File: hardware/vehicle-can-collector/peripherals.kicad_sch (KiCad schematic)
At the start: 16 parts, among them J301 Micro_SD_Card_Det, J302 USB_B_Micro, J303 I2C_STANDARD, U301 FT2232HL, U302 93C56B

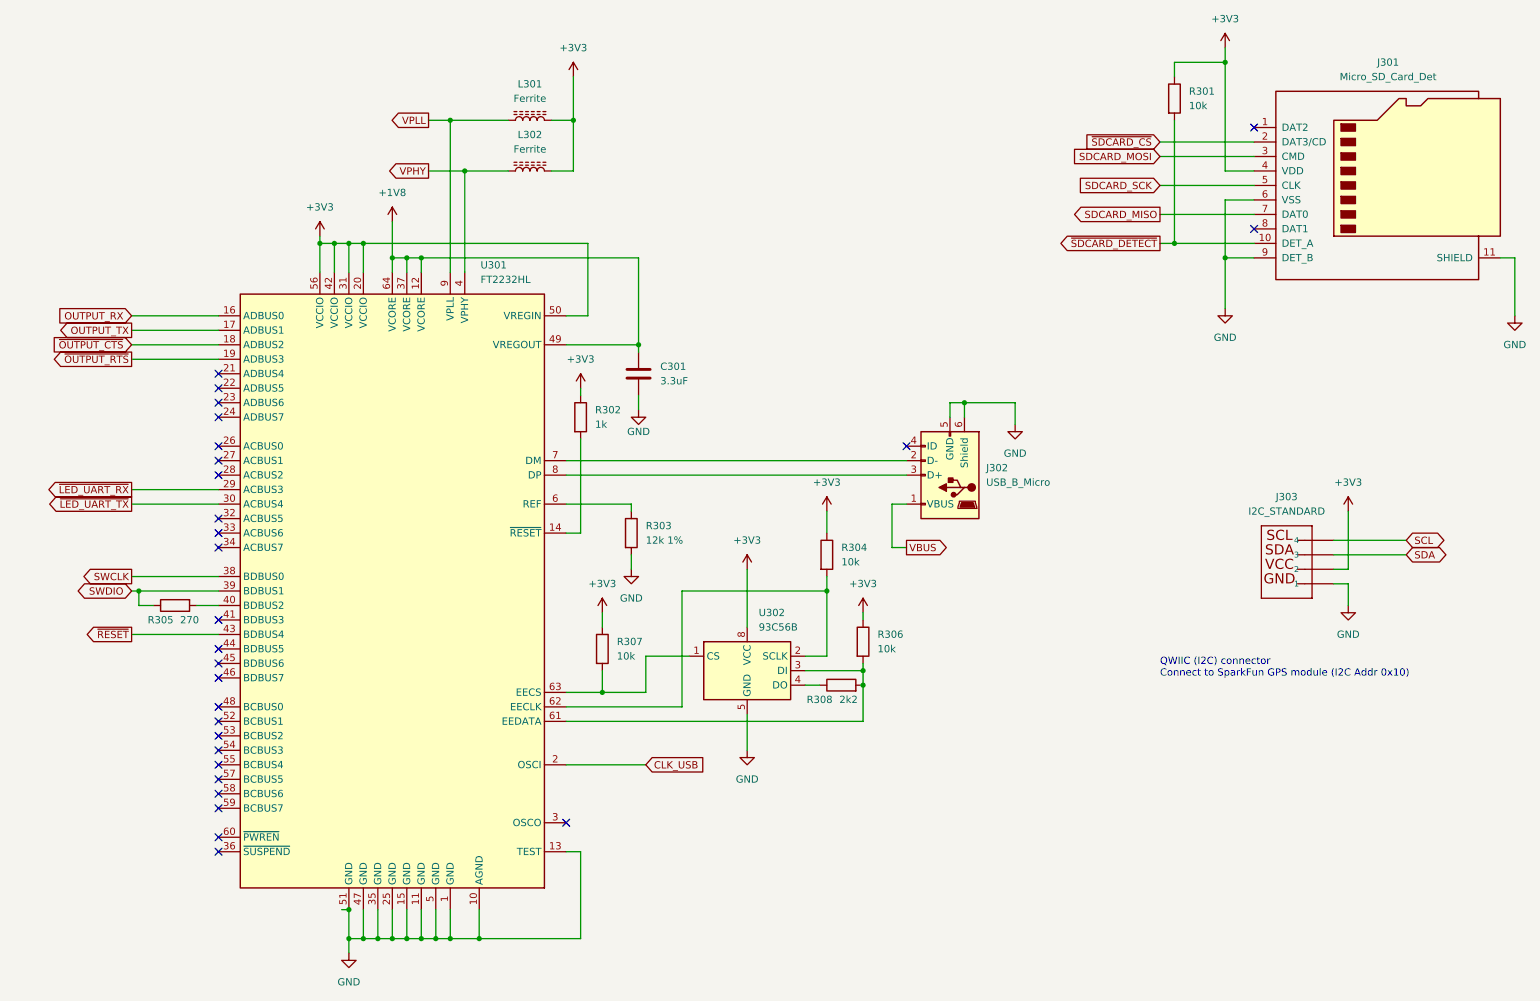
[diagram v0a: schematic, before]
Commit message: Finished first round of layout.
- dang this has a lot of parts!
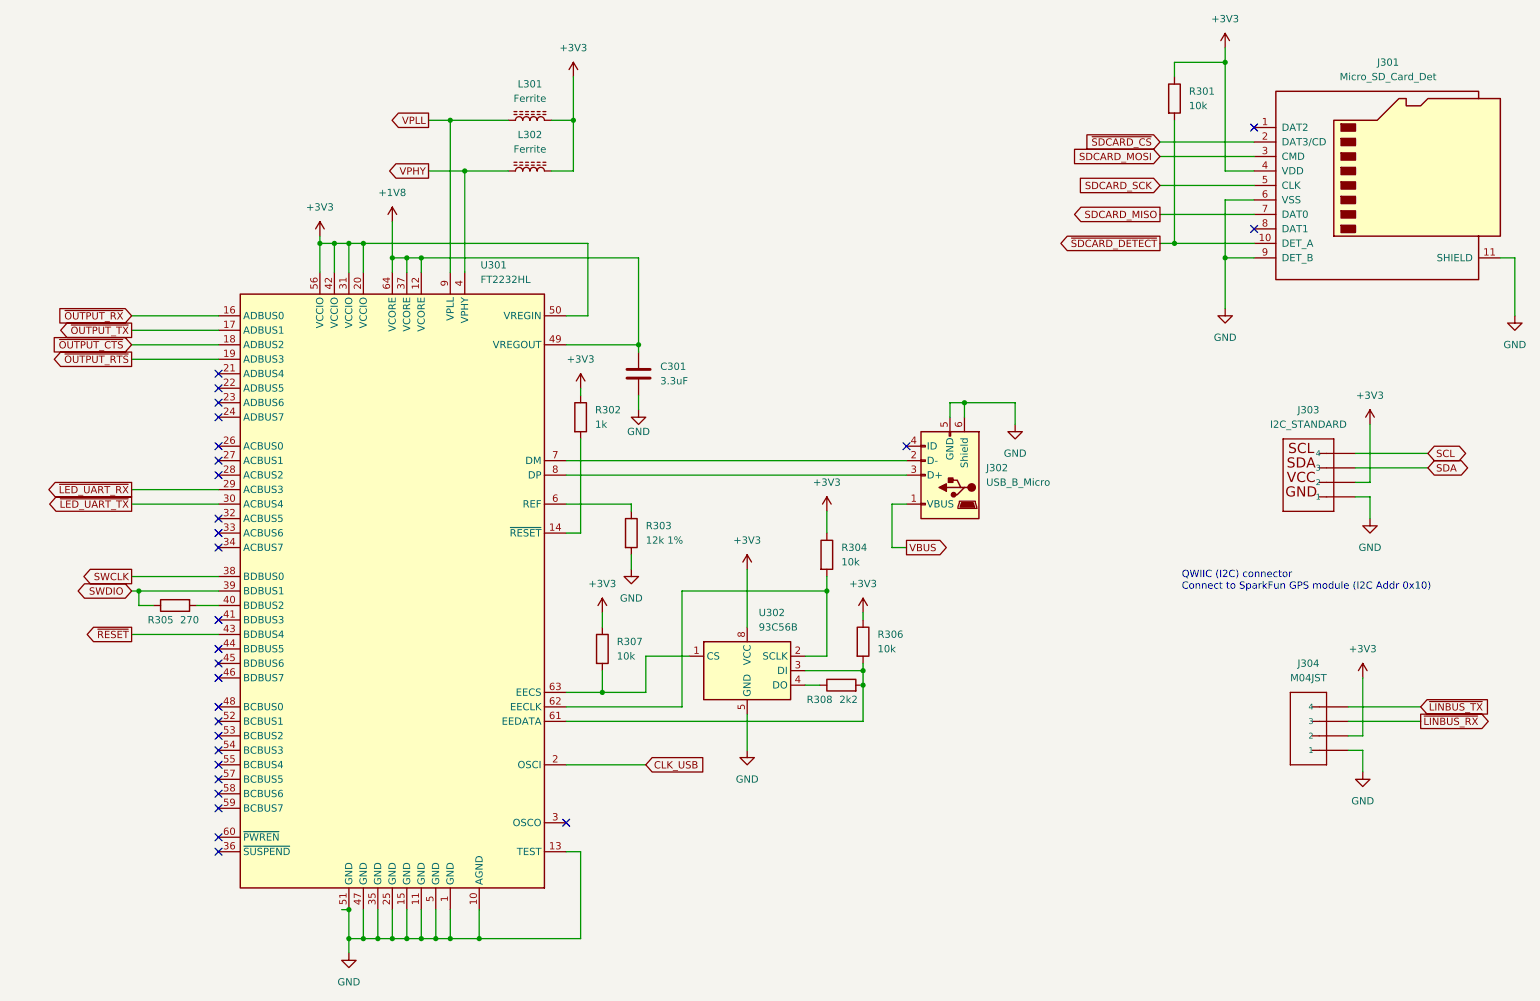
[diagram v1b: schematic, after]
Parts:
- added J304: M04JST, SparkFun-Connectors:1X04-1.5MM_JST, symbol SparkFun-Connectors:M04JST
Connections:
- net +3V3: now also J304.2
- net GND: now also J304.1
- net OUTPUT_RX renamed ~{OUTPUT_RX}
- net OUTPUT_TX renamed ~{OUTPUT_TX}
- new net ~{LINBUS_RX}: J304.3
- new net ~{LINBUS_TX}: J304.4
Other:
- moved on the sheet: J303
